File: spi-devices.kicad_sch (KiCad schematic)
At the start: 27 parts, among them IC5 1v2 LDO, IC6 3v3 LDO, U5 IIM-42652, U8 ICE5LP1K-SG48

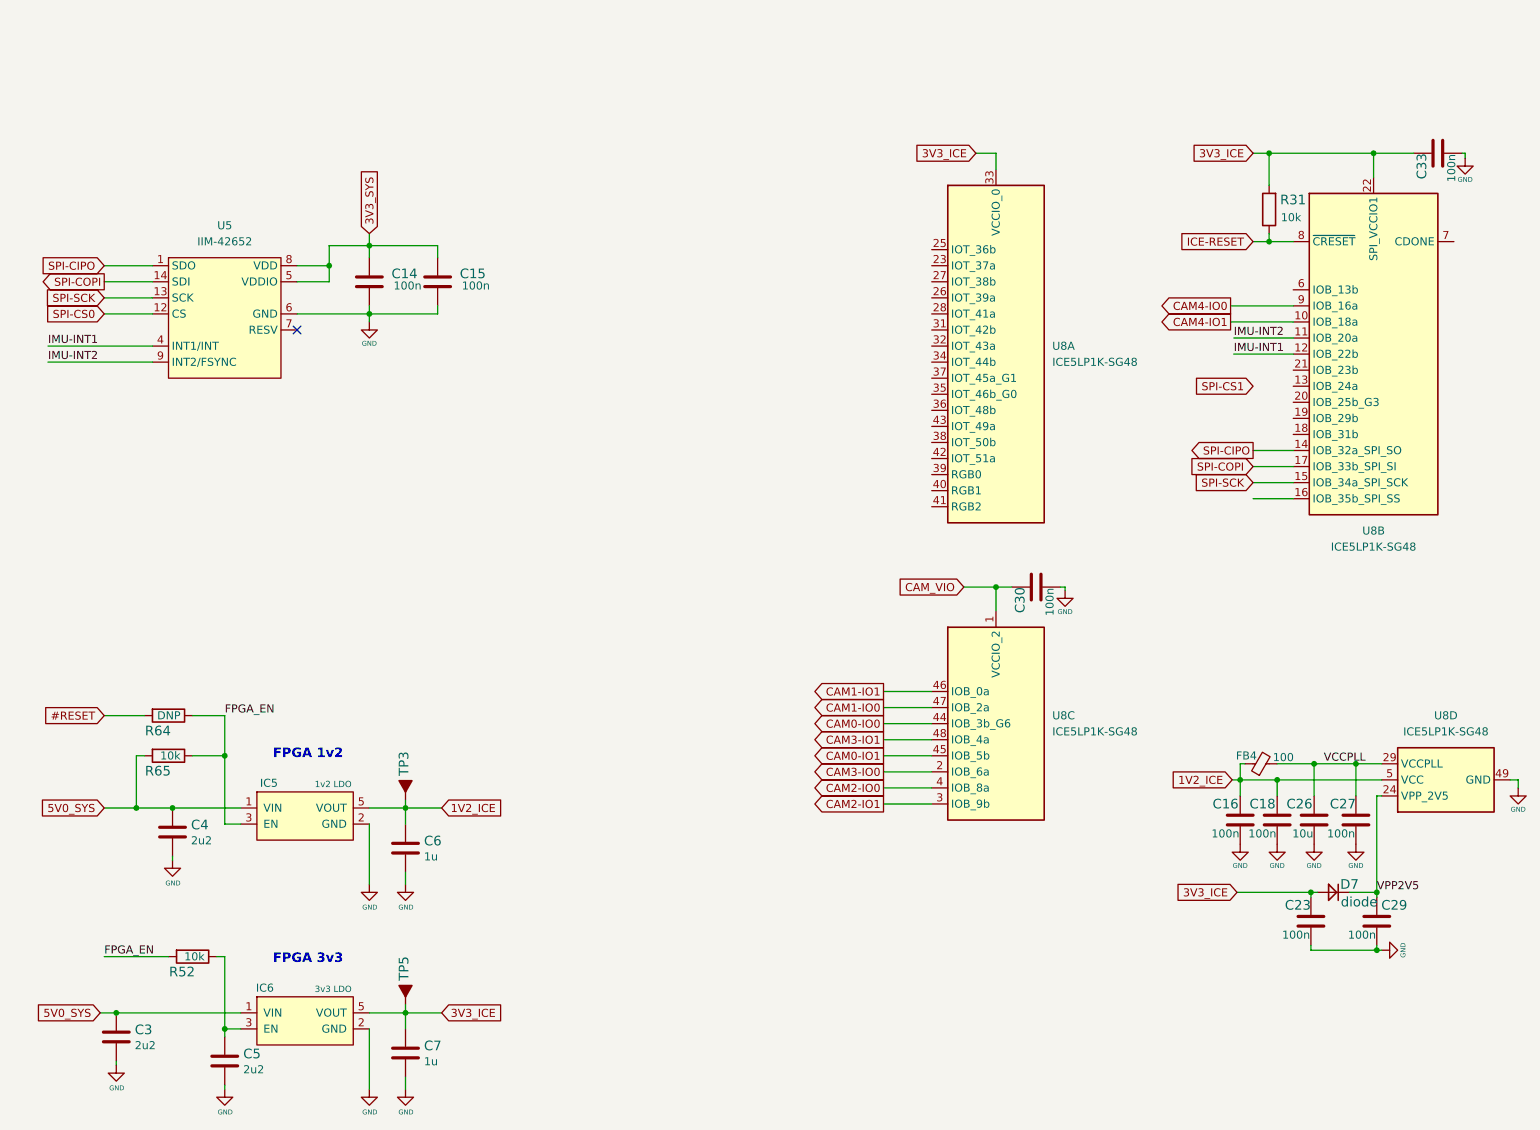
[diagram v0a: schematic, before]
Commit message: Checkpoint
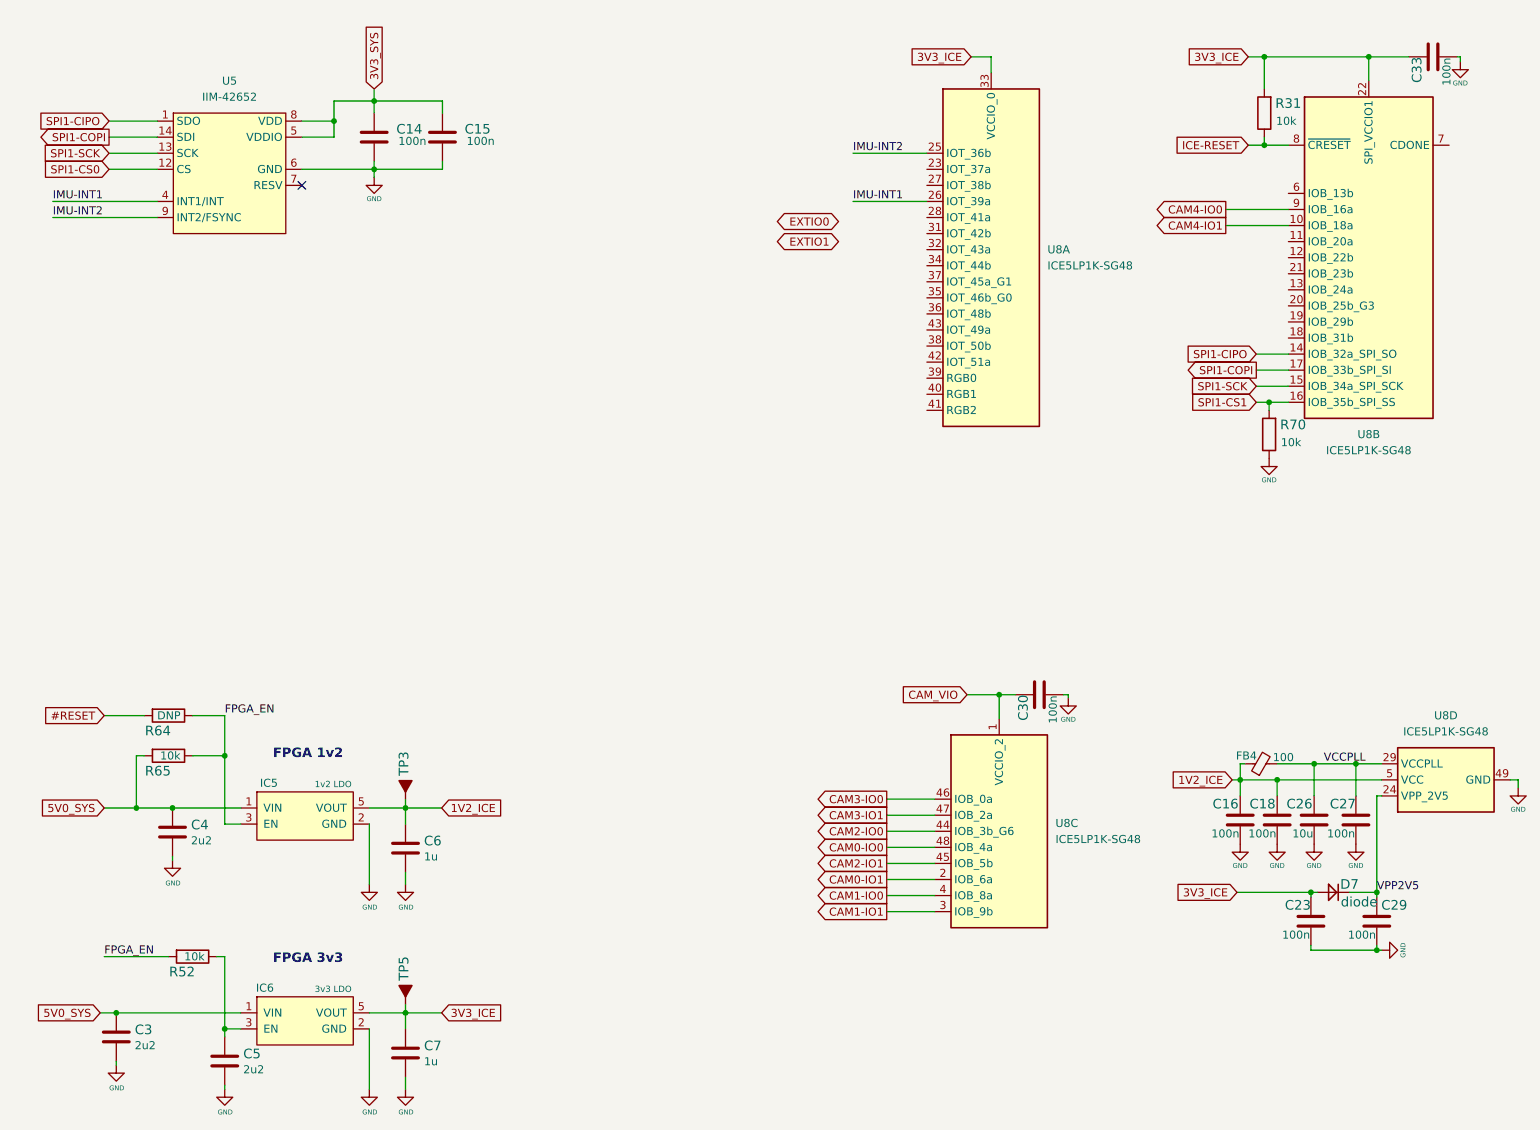
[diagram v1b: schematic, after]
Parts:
- added R70: R_10k_0402, jetson-nano-baseboard-footprints:0402-res, symbol jetson-nano-baseboard:R_10k_0402
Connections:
- net CAM0-IO0: now also U8.48 (IOB_4a); no longer U8.44 (IOB_3b_G6)
- net CAM0-IO1: now also U8.2 (IOB_6a); no longer U8.45 (IOB_5b)
- net CAM1-IO0: now also U8.4 (IOB_8a); no longer U8.47 (IOB_2a)
- net CAM1-IO1: now also U8.3 (IOB_9b); no longer U8.46 (IOB_0a)
- net CAM2-IO0: now also U8.44 (IOB_3b_G6); no longer U8.4 (IOB_8a)
- net CAM2-IO1: now also U8.45 (IOB_5b); no longer U8.3 (IOB_9b)
- net CAM3-IO0: now also U8.46 (IOB_0a); no longer U8.2 (IOB_6a)
- net CAM3-IO1: now also U8.47 (IOB_2a); no longer U8.48 (IOB_4a)
- net GND: now also R70.1
- net IMU-INT1: now also U8.26 (IOT_39a); no longer U8.12 (IOB_22b)
- net IMU-INT2: now also U8.25 (IOT_36b); no longer U8.11 (IOB_20a)
- net SPI1-CS1: now reaches U8.16 (IOB_35b_SPI_SS)
- net SPI1-CS1: now also R70.2
- net SPI-CIPO renamed SPI1-CIPO
- net SPI-COPI renamed SPI1-COPI
- net SPI-CS0 renamed SPI1-CS0
- net SPI-SCK renamed SPI1-SCK
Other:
- moved on the sheet: C14, C15, C30, C33, R31, U5, U8A, U8B, U8C

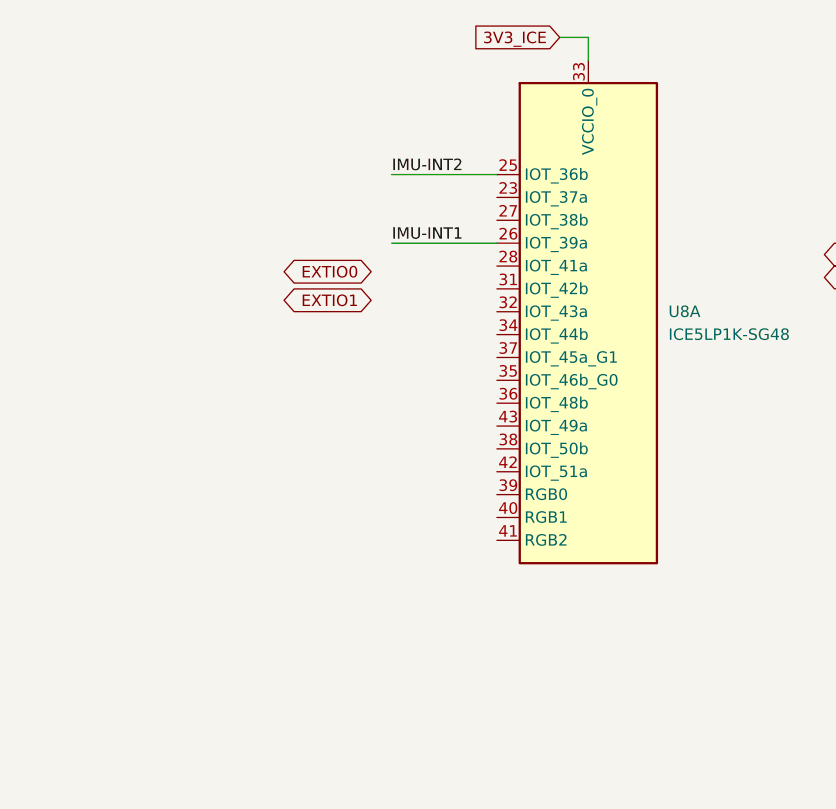
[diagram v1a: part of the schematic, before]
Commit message: Checkpoint
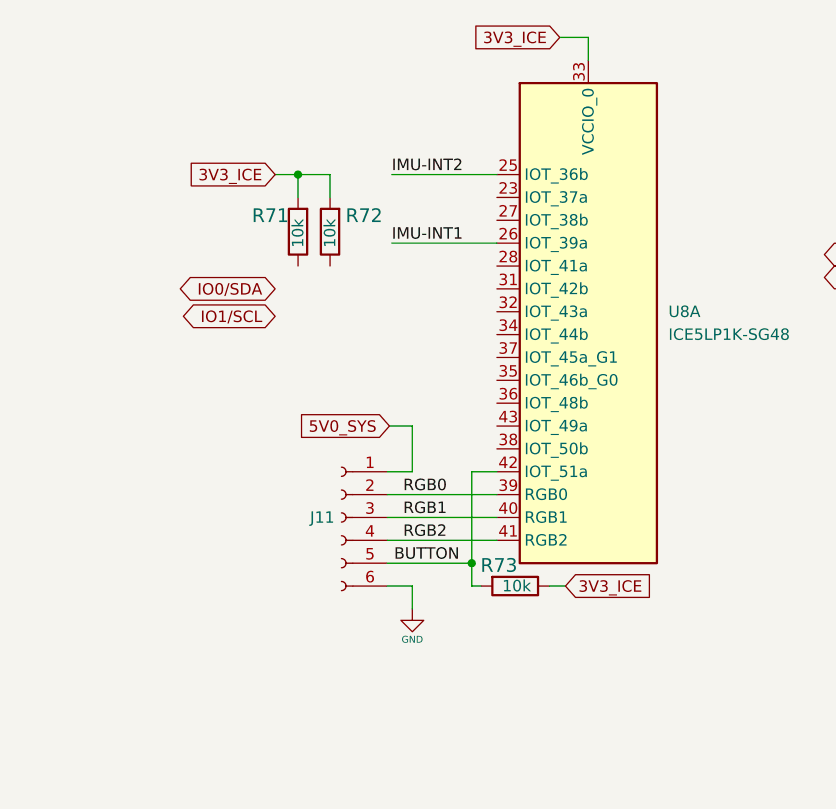
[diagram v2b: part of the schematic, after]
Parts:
- added J11: (no value), symbol Connector:Conn_01x06_Female
- added R71, R72, R73: R_10k_0402, jetson-nano-baseboard-footprints:0402-res, symbol jetson-nano-baseboard:R_10k_0402
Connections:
- net 3V3_ICE: now also R71.2, R72.2, R73.1
- net 5V0_SYS: now also J11.1 (Pin_1)
- net GND: now also J11.6 (Pin_6)
- net RGB0: now reaches U8.39 (RGB0)
- net RGB0: now also J11.2 (Pin_2)
- net RGB1: now reaches U8.40 (RGB1)
- net RGB1: now also J11.3 (Pin_3)
- net RGB2: now reaches U8.41 (RGB2)
- net RGB2: now also J11.4 (Pin_4)
- net BUTTON: now reaches U8.42 (IOT_51a)
- net BUTTON: now also J11.5 (Pin_5), R73.2

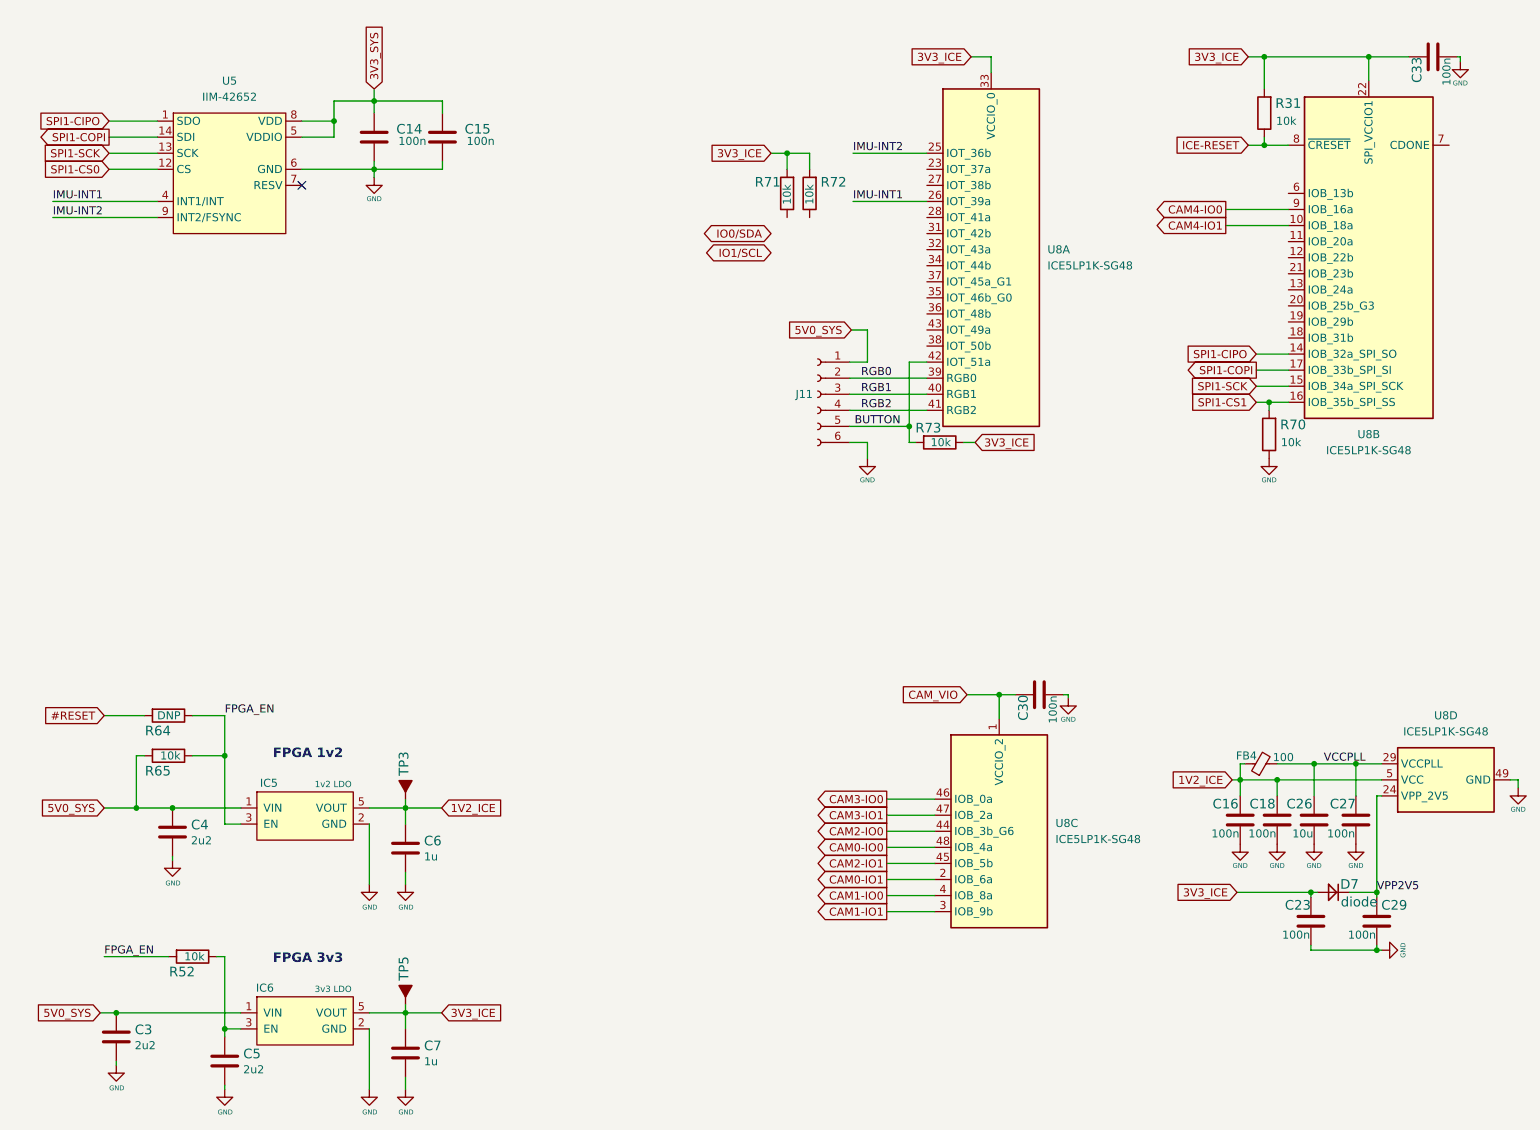
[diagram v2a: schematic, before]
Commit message: Checkpoint
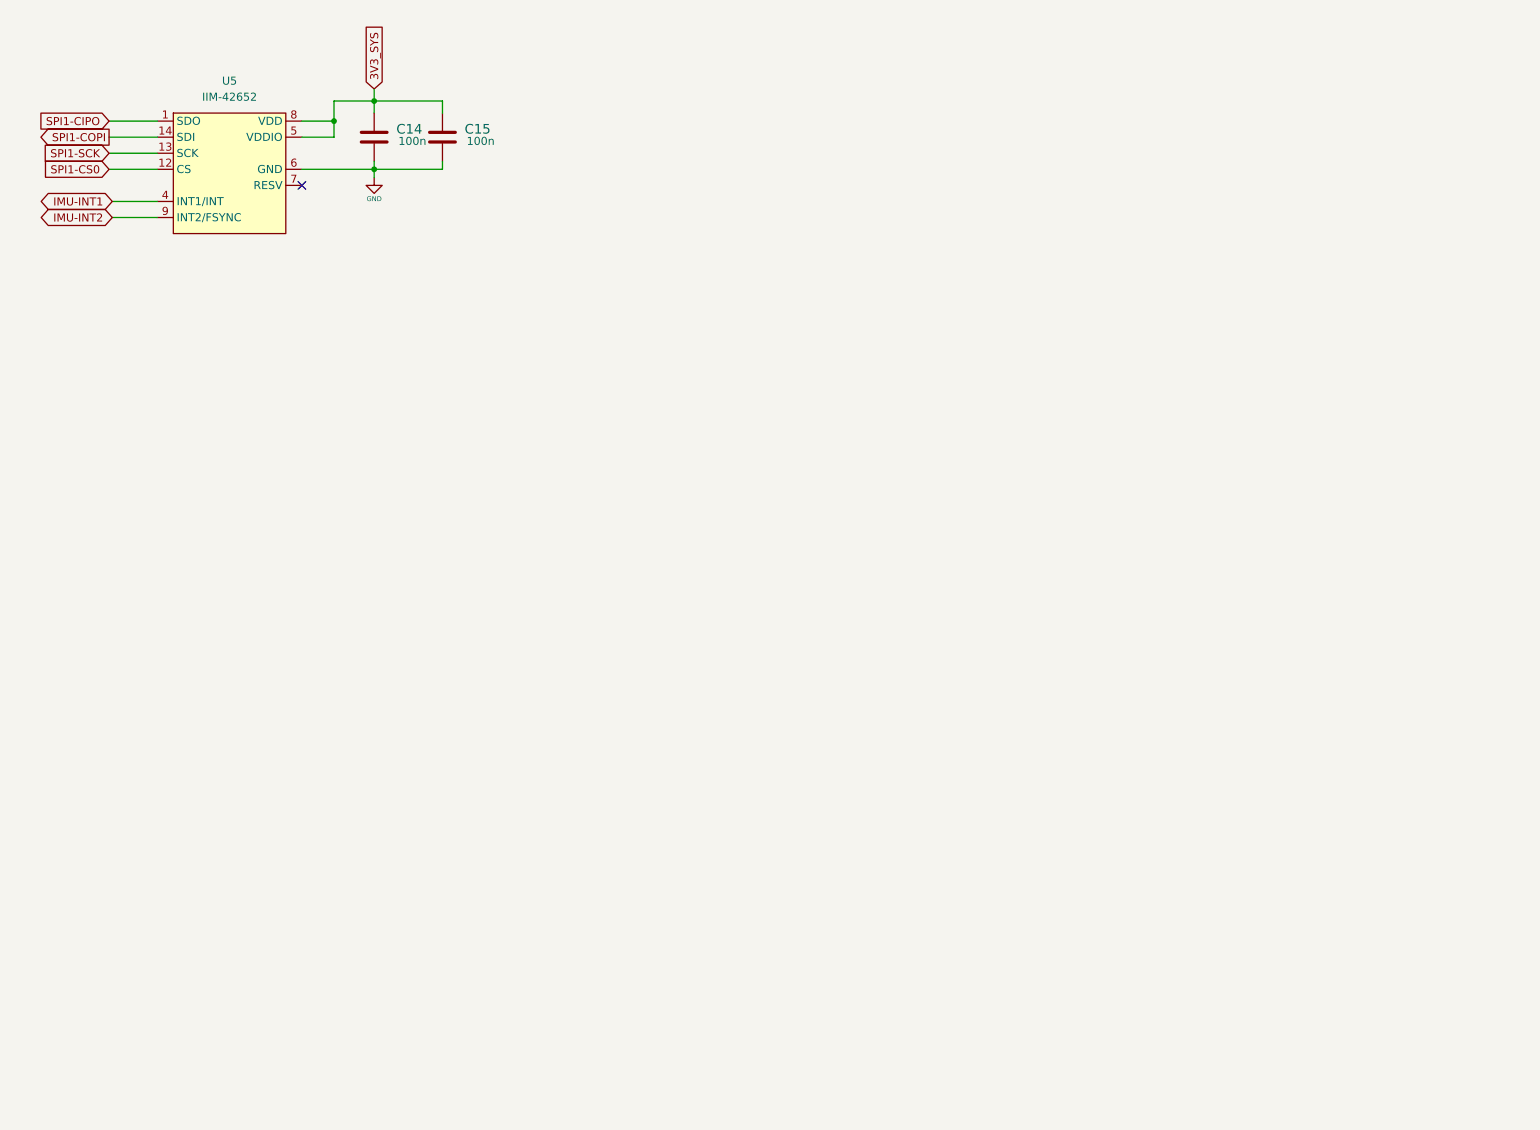
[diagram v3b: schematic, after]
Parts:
- removed C16, C18, C23, C27, C29, C30, C33: C_100n_0402, jetson-nano-baseboard-footprints:0402-cap, symbol jetson-nano-baseboard:C_100n_0402
- removed C26: C_10u_0603, jetson-nano-baseboard-footprints:0603-cap, symbol jetson-nano-baseboard:C_100n_0402
- removed C3, C4, C5: C_2u2_0402, jetson-nano-baseboard-footprints:0402-cap, symbol jetson-nano-baseboard:C_2u2_0402
- removed C6, C7: C_1u_0402, jetson-nano-baseboard-footprints:0402-cap, symbol jetson-nano-baseboard:C_1u_0402
- removed D7: diode, jetson-nano-baseboard-footprints:SOD-323, symbol jetson-nano-baseboard:diode
- removed FB4: 100, jetson-nano-baseboard-footprints:0603-res, symbol Device:FerriteBead_Small
- removed IC5: 1v2 LDO, jetson-nano-baseboard-footprints:SOT-23-5, symbol jetson-nano-baseboard:TPS7A0518PDBVT
- removed IC6: 3v3 LDO, jetson-nano-baseboard-footprints:SOT-23-5, symbol jetson-nano-baseboard:TPS7A0518PDBVT
- removed J11: (no value), symbol Connector:Conn_01x06_Female
- removed R31, R52, R64, R65, R70, R71, R72, R73: R_10k_0402, jetson-nano-baseboard-footprints:0402-res, symbol jetson-nano-baseboard:R_10k_0402
- removed TP3, TP5: ~, jetson-nano-baseboard-footprints:TP-R-1.5, symbol jetson-nano-baseboard:Testpad
- removed U8: ICE5LP1K-SG48, Package_DFN_QFN:QFN-48-1EP_7x7mm_P0.5mm_EP5.6x5.6mm, symbol FPGA_Lattice:ICE5LP1K-SG48
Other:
- note removed: "FPGA 1v2"
- note removed: "FPGA 3v3"
